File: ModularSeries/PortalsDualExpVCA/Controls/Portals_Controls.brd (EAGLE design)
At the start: 48.5 x 100 mm, 15 parts

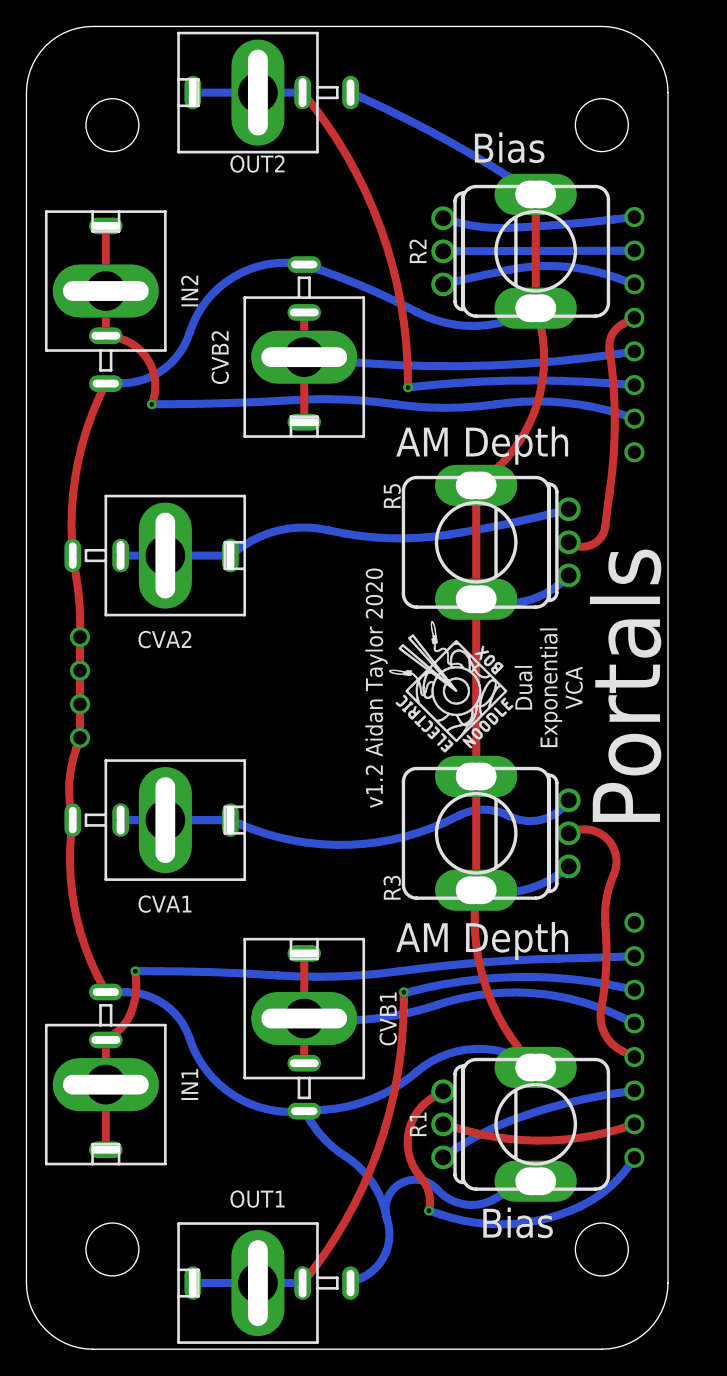
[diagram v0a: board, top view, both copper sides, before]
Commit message: Fields added and various updates to designs
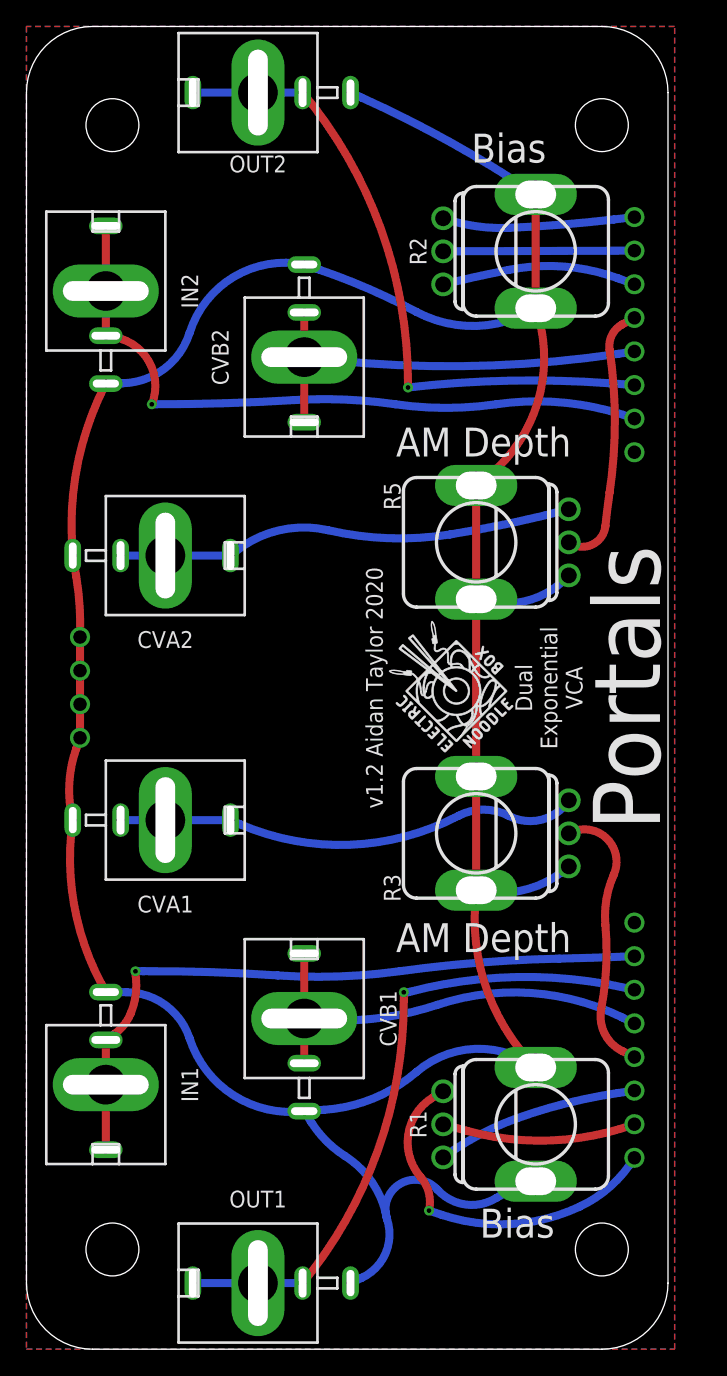
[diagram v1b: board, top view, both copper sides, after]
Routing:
- added copper zone on layer 1, net AGND
- added copper zone on layer 16, net AGND
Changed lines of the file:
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@@
 <setting verticaltext="up"/>
 </settings>
-<grid distance="12.5" unitdist="mil" unit="mil" style="lines" multiple="1" display="no" altdistance="5" altunitdist="mil" altunit="mil"/>
+<grid distance="1" unitdist="mm" unit="mm" style="lines" multiple="1" display="no" altdistance="5" altunitdist="mil" altunit="mil"/>
 <layers>
 <layer number="1" name="Top" color="4" fill="1" visible="yes" active="yes"/>
@@
 <wire x1="8.5725" y1="26.9875" x2="13.335" y2="23.495" width="0.6096" layer="16" curve="-71.596806"/>
 <wire x1="13.335" y1="23.495" x2="22" y2="18" width="0.6096" layer="16" curve="79.341951"/>
+<polygon width="0.5" layer="1">
+<vertex x="1" y="0"/>
+<vertex x="50" y="0"/>
+<vertex x="50" y="100"/>
+<vertex x="1" y="100"/>
+</polygon>
+<polygon width="0.5" layer="16">
+<vertex x="1" y="0"/>
+<vertex x="50" y="0"/>
+<vertex x="50" y="100"/>
+<vertex x="1" y="100"/>
+</polygon>
 </signal>
 <signal name="N$4">
